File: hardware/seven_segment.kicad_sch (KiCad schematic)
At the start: 50 parts, among them J1 Conn_02x08_Odd_Even, J2 PJ-102AH, J3 7761, J4 7761, J5 Conn_01x02, SW1 SW_Push, SW2 SW_Push, SW3 SW_Push, SW4 SW_Push, U1 STM32F051K8Ux, U10 TPS22810DRV, U11 TPS22810DRV, U12 TPS22810DRV, U13 TPS22810DRV, U2 ULN2003A, U3 ULN2003A, U4 AP1117-33, U5 TPS22810DRV, U6 74HC238, U7 TPS22810DRV, U8 TPS22810DRV, U9 TPS22810DRV

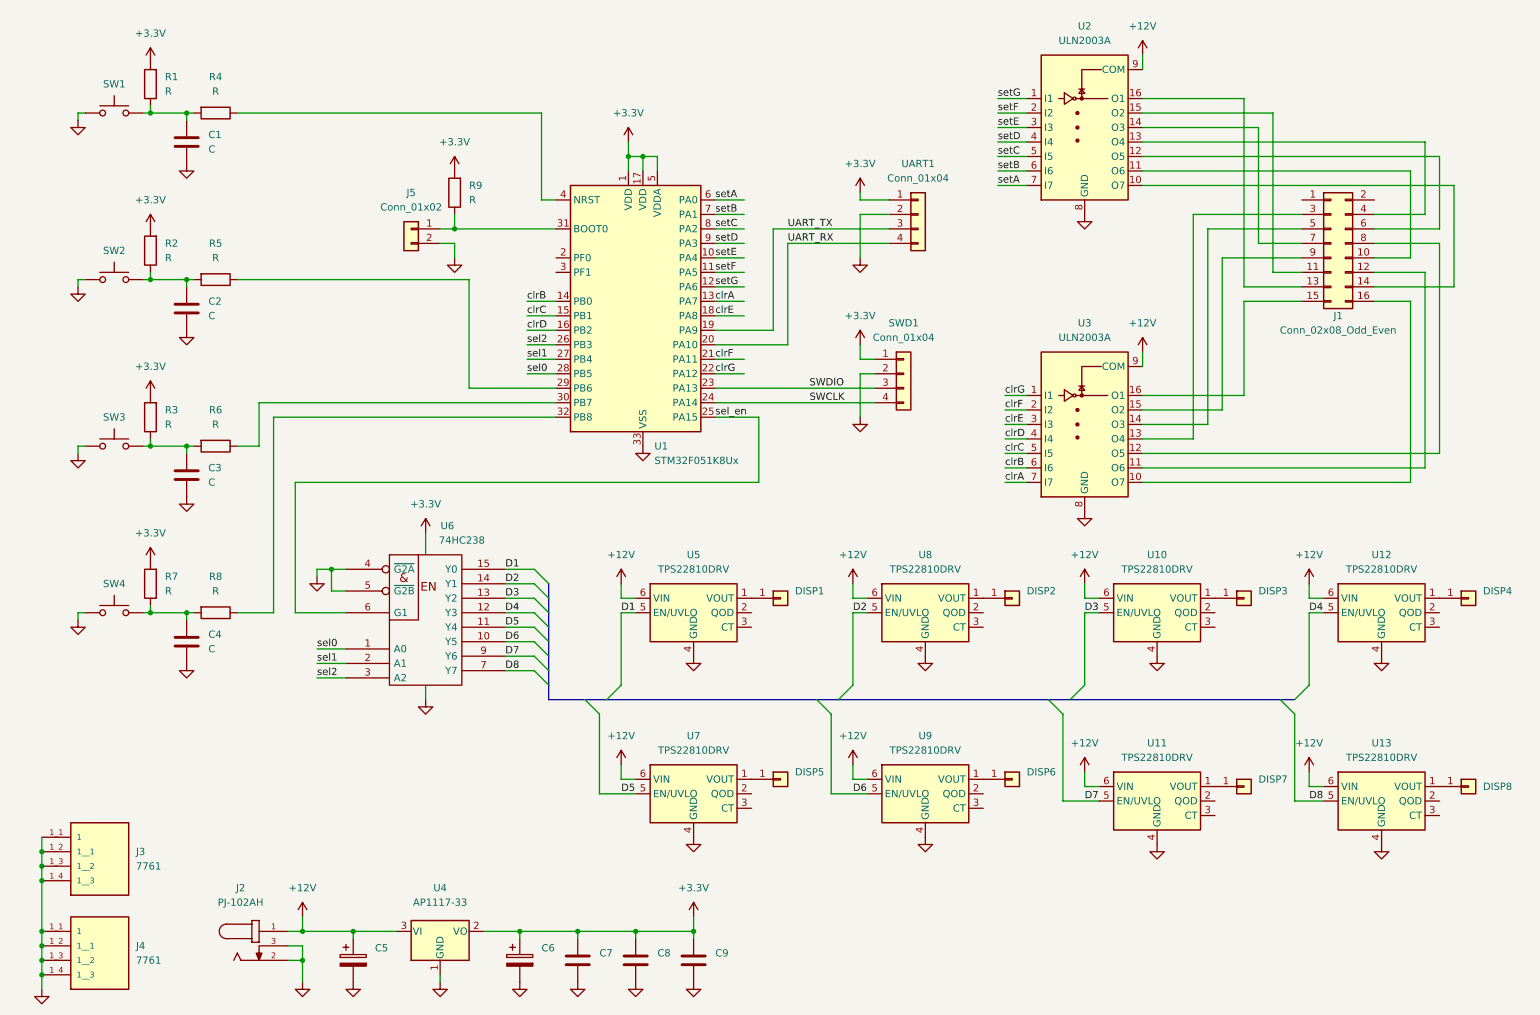
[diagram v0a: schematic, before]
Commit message: hardware: Start work on version 2
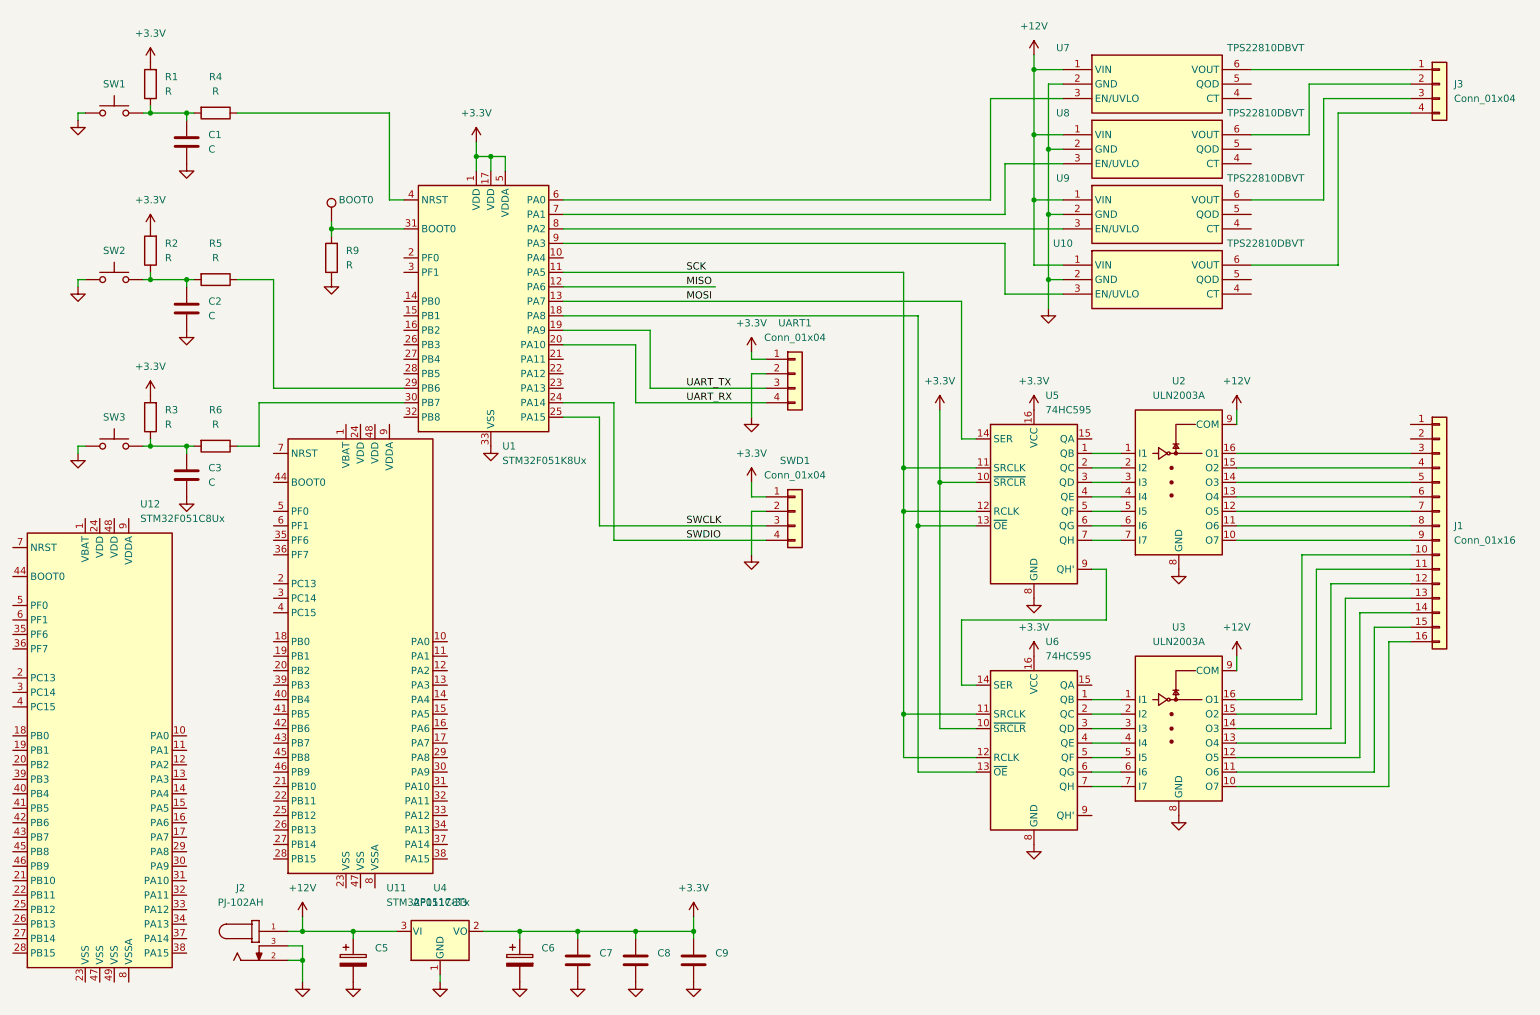
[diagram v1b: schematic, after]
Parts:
- removed C4: C, Resistor_SMD:R_0603_1608Metric, symbol Device:C
- removed DISP1, DISP2, DISP3, DISP4, DISP5, DISP6, DISP7, DISP8: Conn_01x01, klauke:2025, symbol Connector_Generic:Conn_01x01
- removed J1: Conn_02x08_Odd_Even, Connector_PinHeader_2.54mm:PinHeader_2x08_P2.54mm_Horizontal, symbol Connector_Generic:Conn_02x08_Odd_Even
- removed J3, J4: 7761, 7761:KEYSTONE_7761, symbol 7761:7761
- removed J5: Conn_01x02, Connector_PinHeader_2.54mm:PinHeader_1x02_P2.54mm_Vertical, symbol Connector_Generic:Conn_01x02
- removed R7, R8: R, Resistor_SMD:R_0603_1608Metric, symbol Device:R
- removed SW4: SW_Push, pushbutton:TO_6083716_WRE, symbol Switch:SW_Push
- removed U10, U11, U12, U13, U5, U7, U8, U9: TPS22810DRV, Package_SON:WSON-6-1EP_2x2mm_P0.65mm_EP1x1.6mm, symbol Power_Management:TPS22810DRV
- removed U6: 74HC238, Package_SO:SOIC-16W_5.3x10.2mm_P1.27mm, symbol 74xx_IEEE:74HC238
- added BOOT0: BOOT0, TestPoint:TestPoint_Pad_D1.5mm, symbol Connector:TestPoint
- added J1: Conn_01x16, Connector_PinHeader_2.54mm:PinHeader_2x08_P2.54mm_Horizontal, symbol Connector_Generic:Conn_01x16
- added J3: Conn_01x04, Connector_JST:JST_EH_B4B-EH-A_1x04_P2.50mm_Vertical, symbol Connector_Generic:Conn_01x04
- added U10, U7, U8, U9: TPS22810DBVT, Package_TO_SOT_SMD:SOT-23-6, symbol TPS22810DBVT:TPS22810DBVT
- added U11: STM32F051C8Tx, Package_QFP:LQFP-48_7x7mm_P0.5mm, symbol MCU_ST_STM32F0:STM32F051C8Tx
- added U12: STM32F051C8Ux, Package_DFN_QFN:QFN-48-1EP_7x7mm_P0.5mm_EP5.6x5.6mm, symbol MCU_ST_STM32F0:STM32F051C8Ux
- added U5, U6: 74HC595, Package_SO:SOP-16_4.55x10.3mm_P1.27mm, symbol 74xx:74HC595
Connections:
- net sel_en is gone; now on net SWCLK: U1.25 (PA15)
- net +12V: now also U10.1 (VIN), U7.1 (VIN), U8.1 (VIN), U9.1 (VIN)
- net +3V3: now also U5.10 (~{SRCLR}), U5.16 (VCC), U6.10 (~{SRCLR}), U6.16 (VCC); no longer R9.2
- net GND: now also R9.1, U10.2 (GND), U5.8 (GND), U6.8 (GND), U7.2 (GND), U8.2 (GND), U9.2 (GND)
- net SWCLK: now also SWD1.3 (Pin_3); no longer SWD1.4 (Pin_4), U1.24 (PA14)
- net SWDIO: now also SWD1.4 (Pin_4), U1.24 (PA14); no longer SWD1.3 (Pin_3), U1.23 (PA13)
- net at U3.10 (O7): now also J1.16 (Pin_16)
- net at U3.11 (O6): now also J1.15 (Pin_15)
- net at U3.12 (O5): now also J1.14 (Pin_14)
- net at U3.13 (O4): now also J1.13 (Pin_13)
- net at U3.14 (O3): now also J1.12 (Pin_12)
- net at U3.15 (O2): now also J1.11 (Pin_11)
- net at U3.16 (O1): now also J1.10 (Pin_10)
- net at U2.10 (O7): now also J1.9 (Pin_9)
- net at U2.11 (O6): now also J1.8 (Pin_8)
- net at U2.12 (O5): now also J1.7 (Pin_7)
- net at U2.13 (O4): now also J1.6 (Pin_6)
- net at U2.14 (O3): now also J1.5 (Pin_5)
- net at U2.15 (O2): now also J1.4 (Pin_4)
- net at U2.16 (O1): now also J1.3 (Pin_3)
- net at U1.31 (BOOT0): now also R9.2, BOOT0.1; no longer R9.1
- net clrA: no longer names the net of U3.7 (I7)
- net clrA: now also U6.7 (QH); no longer U1.13 (PA7)
- net clrB: no longer names the net of U3.6 (I6)
- net clrB: now also U6.6 (QG); no longer U1.14 (PB0)
- net clrC: no longer names the net of U3.5 (I5)
- net clrC: now also U6.5 (QF); no longer U1.15 (PB1)
- net clrD: no longer names the net of U3.4 (I4)
- net clrD: now also U6.4 (QE); no longer U1.16 (PB2)
- net clrE: no longer names the net of U1.18 (PA8)
- net clrE: now also U5.13 (~{OE}), U6.13 (~{OE}); no longer U3.3 (I3)
- net clrF: no longer names the net of U3.2 (I2)
- net clrF: now also U6.2 (QC); no longer U1.21 (PA11)
- net clrG: no longer names the net of U3.1 (I1)
- net clrG: now also U6.1 (QB); no longer U1.22 (PA12)
- net sel0: no longer names the net of U1.28 (PB5)
- net sel1: no longer names the net of U1.27 (PB4)
- net sel2: no longer names the net of U1.26 (PB3)
- net setA: no longer names the net of U1.6 (PA0)
- net setA: now also U7.3 (EN/UVLO); no longer U2.7 (I7)
- net setB: no longer names the net of U1.7 (PA1)
- net setB: now also U8.3 (EN/UVLO); no longer U2.6 (I6)
- net setC: no longer names the net of U2.5 (I5)
- net setC: now also U5.5 (QF); no longer U1.8 (PA2)
- net setD: no longer names the net of U1.9 (PA3)
- net setD: now also U10.3 (EN/UVLO); no longer U2.4 (I4)
- net setE: no longer names the net of U2.3 (I3)
- net setE: now also U5.3 (QD); no longer U1.10 (PA4)
- net setF: no longer names the net of U2.2 (I2)
- net setF: now also U5.2 (QC); no longer U1.11 (PA5)
- net setG: no longer names the net of U2.1 (I1)
- net setG: now also U5.1 (QB); no longer U1.12 (PA6)
- new net: J3.2 (Pin_2), U8.6 (VOUT)
- new net: J3.4 (Pin_4), U10.6 (VOUT)
- new net: J3.1 (Pin_1), U7.6 (VOUT)
- new net: U2.4 (I4), U5.4 (QE)
- new net: U2.6 (I6), U5.6 (QG)
- new net: U2.7 (I7), U5.7 (QH)
- new net: U5.9 (QH'), U6.14 (SER)
- new net: J3.3 (Pin_3), U9.6 (VOUT)
- new net: U3.3 (I3), U6.3 (QD)
- new net: U1.8 (PA2), U9.3 (EN/UVLO)
- new net MISO: U1.12 (PA6)
- new net MOSI: U1.13 (PA7), U5.14 (SER)
- new net SCK: U1.11 (PA5), U5.11 (SRCLK), U5.12 (RCLK), U6.11 (SRCLK), U6.12 (RCLK)
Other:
- moved on the sheet: R9, SWD1, U1, U2, U3, UART1

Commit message: hardware: Version 2
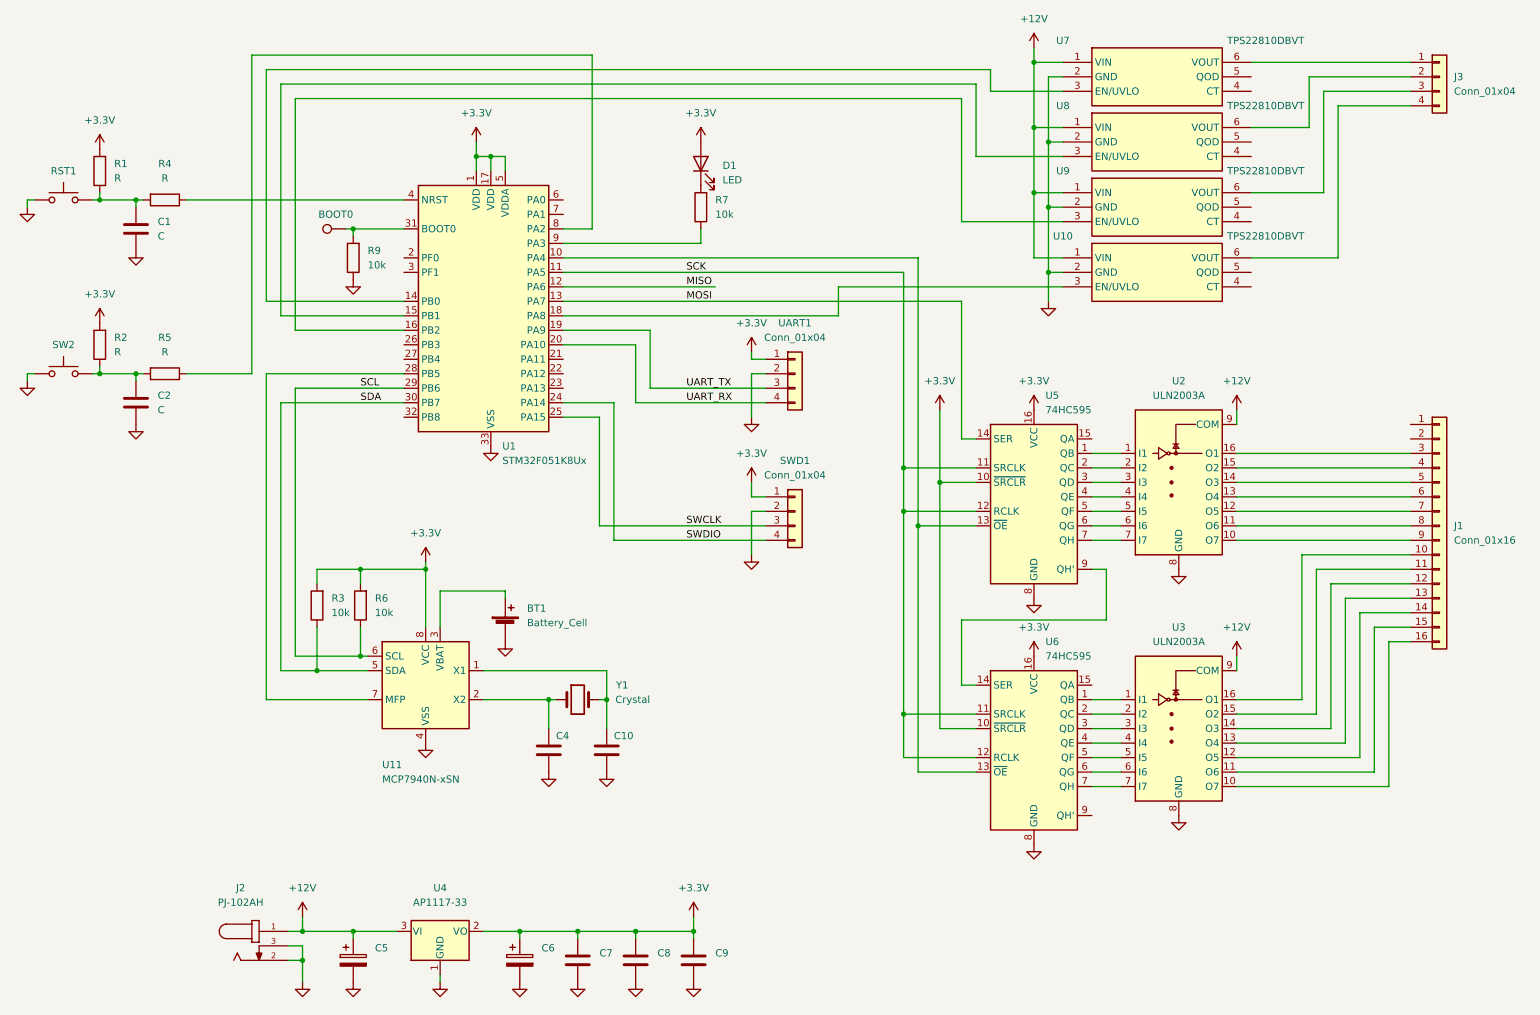
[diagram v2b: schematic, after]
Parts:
- removed C3: C, Resistor_SMD:R_0603_1608Metric, symbol Device:C
- removed SW3: SW_Push, pushbutton:TO_6083716_WRE, symbol Switch:SW_Push
- removed U11: STM32F051C8Tx, Package_QFP:LQFP-48_7x7mm_P0.5mm, symbol MCU_ST_STM32F0:STM32F051C8Tx
- removed U12: STM32F051C8Ux, Package_DFN_QFN:QFN-48-1EP_7x7mm_P0.5mm_EP5.6x5.6mm, symbol MCU_ST_STM32F0:STM32F051C8Ux
- added BT1: Battery_Cell, Battery:BatteryHolder_Keystone_3000_1x12mm, symbol Device:Battery_Cell
- added C10, C4: C, Resistor_SMD:R_0402_1005Metric_Pad0.72x0.64mm_HandSolder, symbol Device:C
- added D1: LED, Connector_PinHeader_2.54mm:PinHeader_1x02_P2.54mm_Vertical, symbol Device:LED
- added R7: 10k, Resistor_SMD:R_0603_1608Metric, symbol Device:R
- added U11: MCP7940N-xSN, Package_SO:SO-8_3.9x4.9mm_P1.27mm, symbol Timer_RTC:MCP7940N-xSN
- added Y1: Crystal, Crystal:Crystal_SMD_3215-2Pin_3.2x1.5mm, symbol Device:Crystal
- C5, C6: footprint Capacitor_THT:CP_Radial_D7.5mm_P2.50mm -> Capacitor_SMD:CP_Elec_6.3x5.9
- R3, R6, R9: value R -> 10k
- renumbered SW1 to RST1
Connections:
- net +3V3: now also R6.2, D1.2 (A), U11.8 (VCC)
- net GND: now also BT1.2 (-), C10.2, C4.2, U11.4 (VSS)
- net at U8.3 (EN/UVLO): now also U1.15 (PB1); no longer U1.7 (PA1)
- net SDA: now reaches R3.1
- net SDA: now also U1.30 (PB7), U11.5 (SDA); no longer R6.2
- net at U10.3 (EN/UVLO): now also U1.18 (PA8); no longer U1.9 (PA3)
- net at U7.3 (EN/UVLO): now also U1.14 (PB0); no longer U1.6 (PA0)
- net at U5.13 (~{OE}), U6.13 (~{OE}): now also U1.10 (PA4); no longer U1.18 (PA8)
- net at R5.1: now also U1.8 (PA2); no longer U1.29 (PB6)
- net at U9.3 (EN/UVLO): now also U1.16 (PB2); no longer U1.8 (PA2)
- net SCL: now reaches R6.1
- net SCL: now also U1.29 (PB6), U11.6 (SCL); no longer U1.30 (PB7)
- net at U1.28 (PB5): now also U11.7 (MFP)
- new net: C10.1, U11.1 (X1), Y1.2
- new net: C4.1, U11.2 (X2), Y1.1
- new net: BT1.1 (+), U11.3 (VBAT)
- new net: D1.1 (K), R7.2
- new net: R7.1, U1.9 (PA3)
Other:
- moved on the sheet: BOOT0, C1, C2, J3, R1, R2, R4, R5, R9, RST1, SW2, U10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
